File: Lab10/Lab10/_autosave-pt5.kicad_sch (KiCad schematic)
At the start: 15 parts, among them U7 LM339, U8 LM324, U9 uA7812

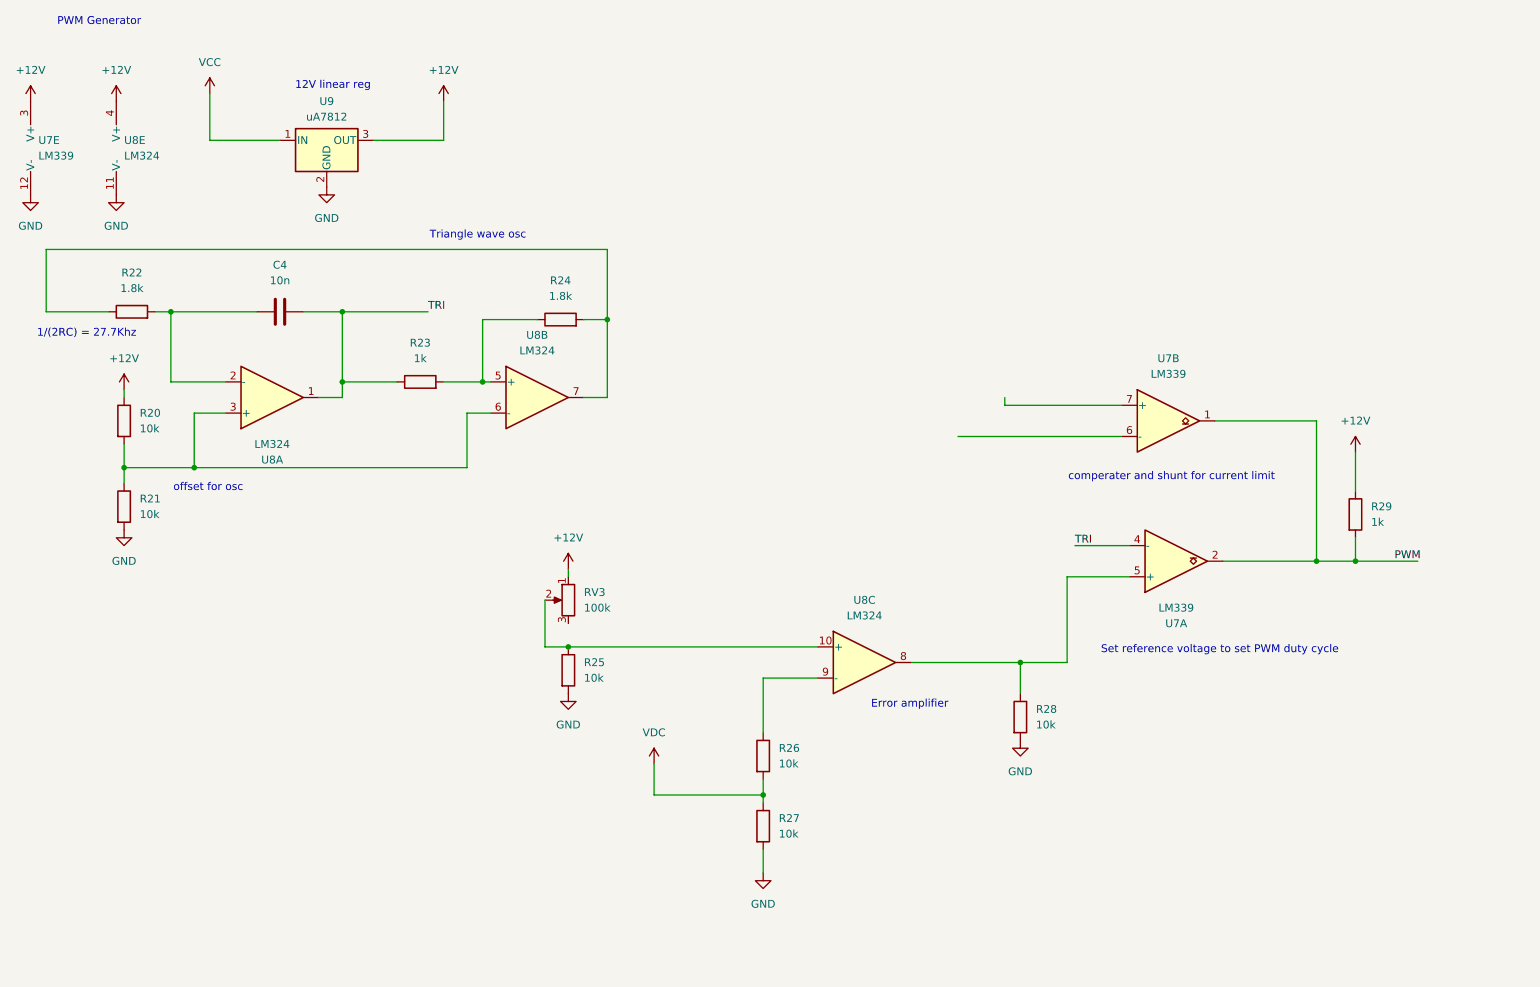
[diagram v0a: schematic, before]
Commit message: 3ab11
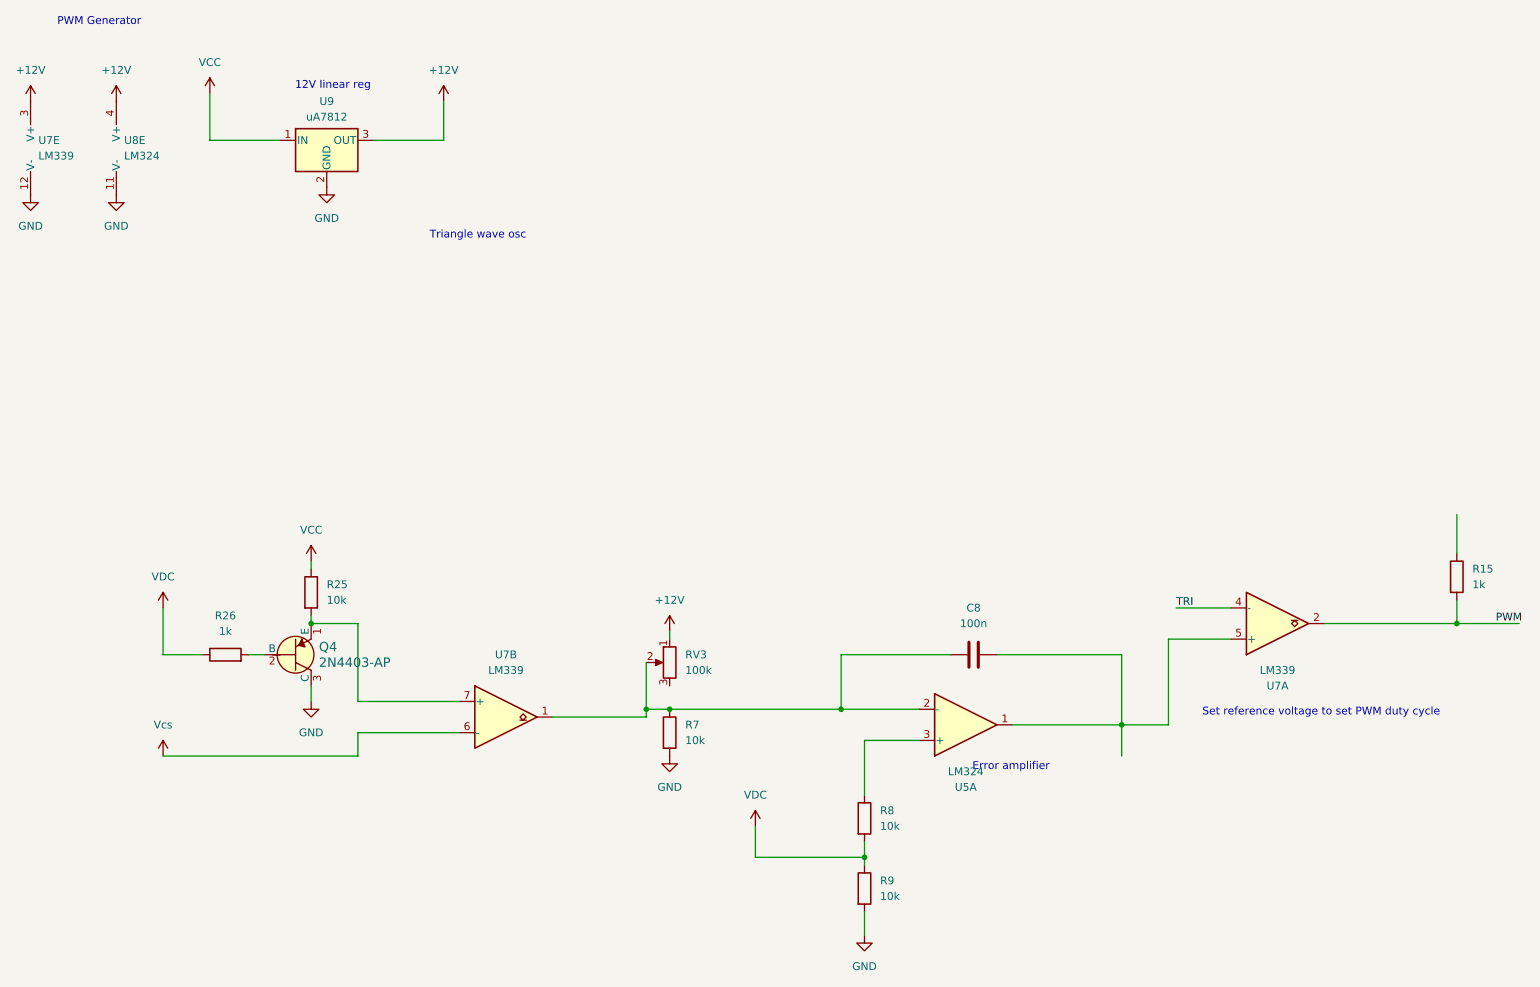
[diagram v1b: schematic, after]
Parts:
- removed C4: 10n, symbol Device:C
- removed R20, R21, R27, R28: 10k, symbol Device:R
- removed R22, R24: 1.8k, symbol Device:R
- removed R23, R29: 1k, symbol Device:R
- removed unit 1 of U8
- removed unit 2 of U8
- removed unit 3 of U8
- added C8: 100n, symbol Device:C
- added Q4: 2N4403-AP, digikey-footprints:TO-92-3_Formed_Leads, symbol dk_Transistors-Bipolar-BJT-Single:2N4403-AP
- added R15: 1k, symbol Device:R
- added R7, R8, R9: 10k, symbol Device:R
- added U5: LM324, symbol Amplifier_Operational:LM324
- R26: value 10k -> 1k
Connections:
- net GND: now also Q4.3 (C), R7.2, R9.2; no longer R25.2
- net PWM: now also R15.2; no longer U7.1
- net VCC: now also R25.1
- net VDC: now also R26.1, R8.2, R9.1; no longer R26.2
- net at RV3.2: now also U7.1, C8.1, R7.1, U5.2 (-); no longer R25.1
- net at U7.5 (+): now also C8.2, U5.1
- net Vcs: now reaches U7.6 (-)
- net at U7.7 (+): now also R25.2, Q4.1 (E)
- new net: R8.1, U5.3 (+)
- new net: Q4.2 (B), R26.2
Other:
- note removed: "1/(2RC) = 27.7Khz"
- note removed: "comperater and shunt for current limit"
- note removed: "offset for osc"
